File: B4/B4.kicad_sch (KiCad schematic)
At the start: 0 parts

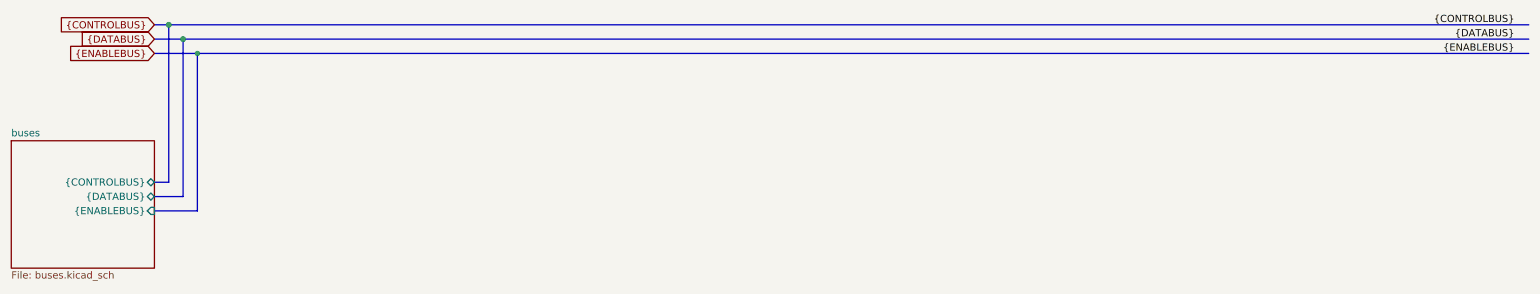
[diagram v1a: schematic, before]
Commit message: B0 ready for v0.2.0 release.
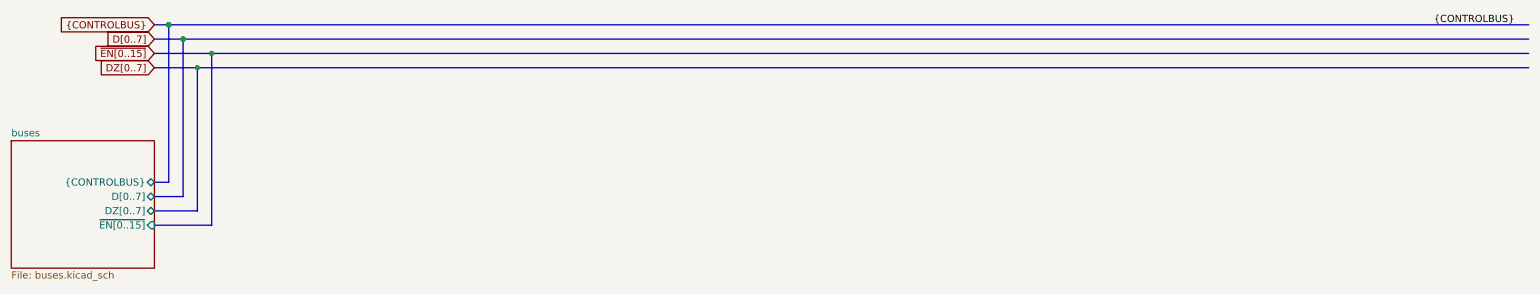
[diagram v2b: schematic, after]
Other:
- sheet buses ports: added DZ[0..7], D[0..7], ~{EN[0..15]}; removed {DATABUS}, {ENABLEBUS}
- company: (none) -> Daniel Molina
- title: (none) -> 74HCT6526 Board 4
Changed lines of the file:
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@@
 (kicad_sch (version 20211123) (generator eeschema)
   (paper "A4")
+  (title_block
+    (title "74HCT6526 Board 4")
+    (date "2023-01-22")
+    (rev "0.2.0")
+    (company "Daniel Molina")
+    (comment 1 "https://github.com/dmolinagarcia/74HCT6526")
+  )
   (bus_alias "ENABLEBUS" (members "~{EN[0..15]}"))
   (bus_alias "DATABUS" (members "D[0..7]" "DZ[0..7]"))
@@
   (junction (at 43.18 17.78) (diameter 1.016) (color 0 0 0 0)
   )
-  (junction (at 48.26 22.86) (diameter 0.9144) (color 0 0 0 0)
+  (junction (at 48.26 25.4) (diameter 0) (color 0 0 0 0)
+  )
+  (junction (at 50.8 22.86) (diameter 0) (color 0 0 0 0)
   )
   (junction (at 45.72 20.32) (diameter 1.016) (color 0 0 0 0)
@@
     (stroke (width 0) (type solid) (color 0 0 0 0))
   )
+  (bus (pts (xy 48.26 50.8) (xy 48.26 25.4))
+    (stroke (width 0) (type default) (color 0 0 0 0))
+  )
   (bus (pts (xy 43.18 17.78) (xy 284.48 17.78))
     (stroke (width 0) (type solid) (color 0 0 0 0))
   )
-  (bus (pts (xy 40.64 50.8) (xy 48.26 50.8))
+  (bus (pts (xy 40.64 53.34) (xy 50.8 53.34))
     (stroke (width 0) (type solid) (color 0 0 0 0))
   )
@@
     (stroke (width 0) (type solid) (color 0 0 0 0))
   )
-  (bus (pts (xy 48.26 50.8) (xy 48.26 22.86))
+  (bus (pts (xy 50.8 53.34) (xy 50.8 22.86))
     (stroke (width 0) (type solid) (color 0 0 0 0))
   )
   (bus (pts (xy 40.64 45.72) (xy 43.18 45.72))
     (stroke (width 0) (type solid) (color 0 0 0 0))
+  )
+  (bus (pts (xy 48.26 25.4) (xy 284.48 25.4))
+    (stroke (width 0) (type default) (color 0 0 0 0))
+  )
+  (bus (pts (xy 40.64 25.4) (xy 48.26 25.4))
+    (stroke (width 0) (type default) (color 0 0 0 0))
+  )
+  (bus (pts (xy 40.64 50.8) (xy 48.26 50.8))
+    (stroke (width 0) (type default) (color 0 0 0 0))
   )
   (bus (pts (xy 43.18 17.78) (xy 43.18 45.72))
@@
     (stroke (width 0) (type solid) (color 0 0 0 0))
   )
-  (bus (pts (xy 40.64 22.86) (xy 48.26 22.86))
+  (bus (pts (xy 40.64 22.86) (xy 50.8 22.86))
     (stroke (width 0) (type solid) (color 0 0 0 0))
   )
-  (bus (pts (xy 48.26 22.86) (xy 284.48 22.86))
+  (bus (pts (xy 50.8 22.86) (xy 284.48 22.86))
     (stroke (width 0) (type solid) (color 0 0 0 0))
   )
@@
     (stroke (width 0) (type solid) (color 0 0 0 0))
   )
-  (label "{DATABUS}" (at 281.94 20.32 180)
-    (effects (font (size 1.27 1.27)) (justify right bottom))
-  )
-  (label "{ENABLEBUS}" (at 281.94 22.86 180)
-    (effects (font (size 1.27 1.27)) (justify right bottom))
-  )
   (label "{CONTROLBUS}" (at 281.94 17.78 180)
     (effects (font (size 1.27 1.27)) (justify right bottom))
   )
-  (global_label "{DATABUS}" (shape input) (at 40.64 20.32 180)
+  (global_label "D[0..7]" (shape input) (at 40.64 20.32 180)
     (effects (font (size 1.27 1.27)) (justify right))
     (property "Intersheet References" "${INTERSHEET_REFS}" (id 0) (at 26.7848 20.2406 0)
@@
     )
   )
-  (global_label "{ENABLEBUS}" (shape input) (at 40.64 22.86 180)
+  (global_label "~{EN[0..15]}" (shape input) (at 40.64 22.86 180)
     (effects (font (size 1.27 1.27)) (justify right))
     (property "Intersheet References" "${INTERSHEET_REFS}" (id 0) (at 24.1843 22.7806 0)
@@
     (effects (font (size 1.27 1.27)) (justify right))
     (property "Intersheet References" "${INTERSHEET_REFS}" (id 0) (at 22.6724 17.7006 0)
+      (effects (font (size 1.27 1.27)) (justify right) hide)
+    )
+  )
+  (global_label "DZ[0..7]" (shape input) (at 40.64 25.4 180)
+    (effects (font (size 1.27 1.27)) (justify right))
+    (property "Intersheet References" "${INTERSHEET_REFS}" (id 0) (at 26.7848 25.3206 0)
       (effects (font (size 1.27 1.27)) (justify right) hide)
     )
@@
       (effects (font (size 1.27 1.27)) (justify right))
     )
-    (pin "{DATABUS}" bidirectional (at 40.64 48.26 0)
+    (pin "D[0..7]" bidirectional (at 40.64 48.26 0)
       (effects (font (size 1.27 1.27)) (justify right))
     )
-    (pin "{ENABLEBUS}" input (at 40.64 50.8 0)
+    (pin "~{EN[0..15]}" input (at 40.64 53.34 0)
+      (effects (font (size 1.27 1.27)) (justify right))
+    )
+    (pin "DZ[0..7]" bidirectional (at 40.64 50.8 0)
       (effects (font (size 1.27 1.27)) (justify right))
     )
@@
       (reference "#PWR04") (unit 1) (value "GND") (footprint "")
     )
+    (path "/ab70af84-b545-4f99-8702-a579edb051a6/8554bcb8-444f-4ed6-8d2e-98ad945f68d5"
+      (reference "#PWR?") (unit 1) (value "GND") (footprint "")
+    )
+    (path "/ab70af84-b545-4f99-8702-a579edb051a6/989f85db-f560-481a-baba-d8c4193b2250"
+      (reference "C400") (unit 1) (value "100n") (footprint "")
+    )
     (path "/ab70af84-b545-4f99-8702-a579edb051a6/eb77a2b8-05ae-49a3-b81c-407677587e70"

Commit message: Ready for v0.2.1
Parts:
- added U401, U402: 74HC00, symbol 74xx:74HC00
- added U403: 74HC04, Package_SO:SOIC-14_3.9x8.7mm_P1.27mm, symbol 74xx:74HC04
- added U404, U405, U406: 74HC32, symbol 74xx:74LS32
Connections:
- new net PHI2: U403.1
- new net ~{PHI2}: U403.2
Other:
- added sheet todAlarm (todAlarm.kicad_sch)
- added sheet todComparator (todComparator.kicad_sch)
- added sheet todControl (todControl.kicad_sch)
- added sheet todCounter (todCounter.kicad_sch)
- added sheet todOutput (todOutput.kicad_sch)
